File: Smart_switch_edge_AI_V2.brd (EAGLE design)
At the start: 60.6 x 40.8 mm, 13 parts, among them K1 AQG12105, K2 AQG12105, K3 AQG12105

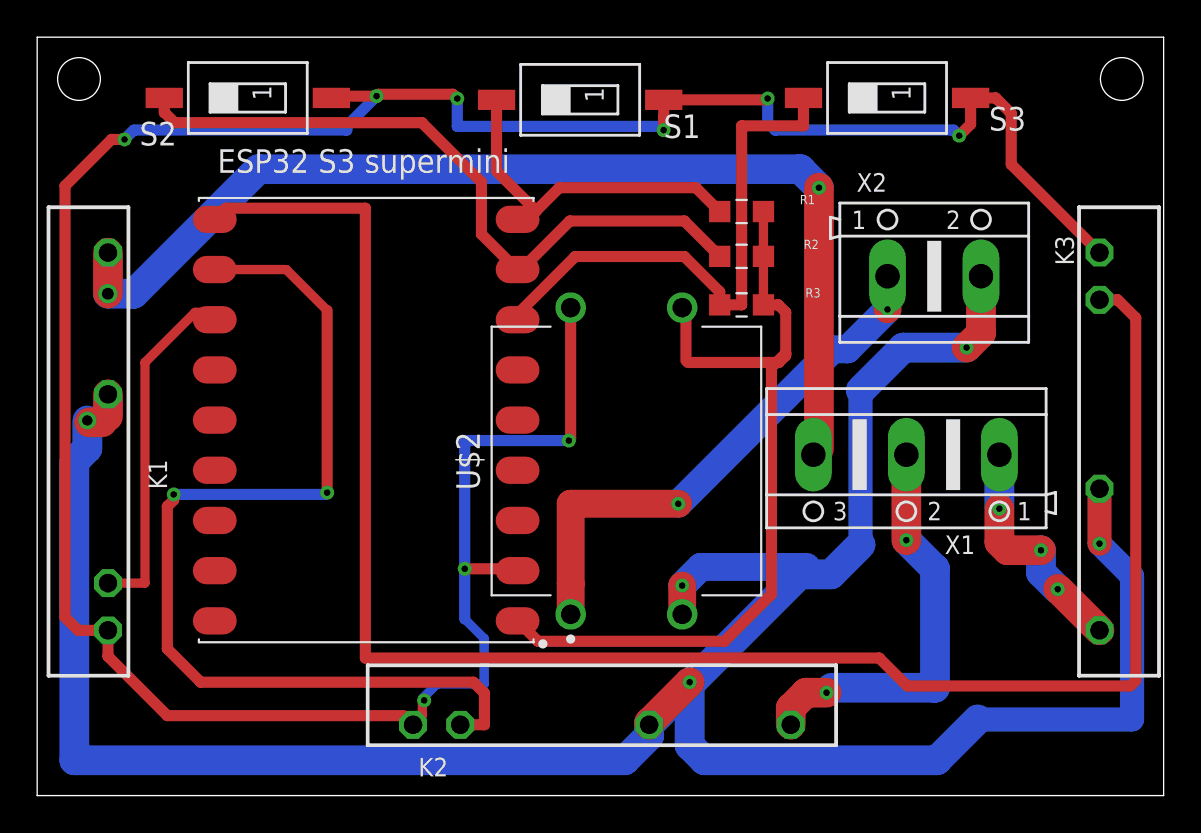
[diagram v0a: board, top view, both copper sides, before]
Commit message: Add files via upload
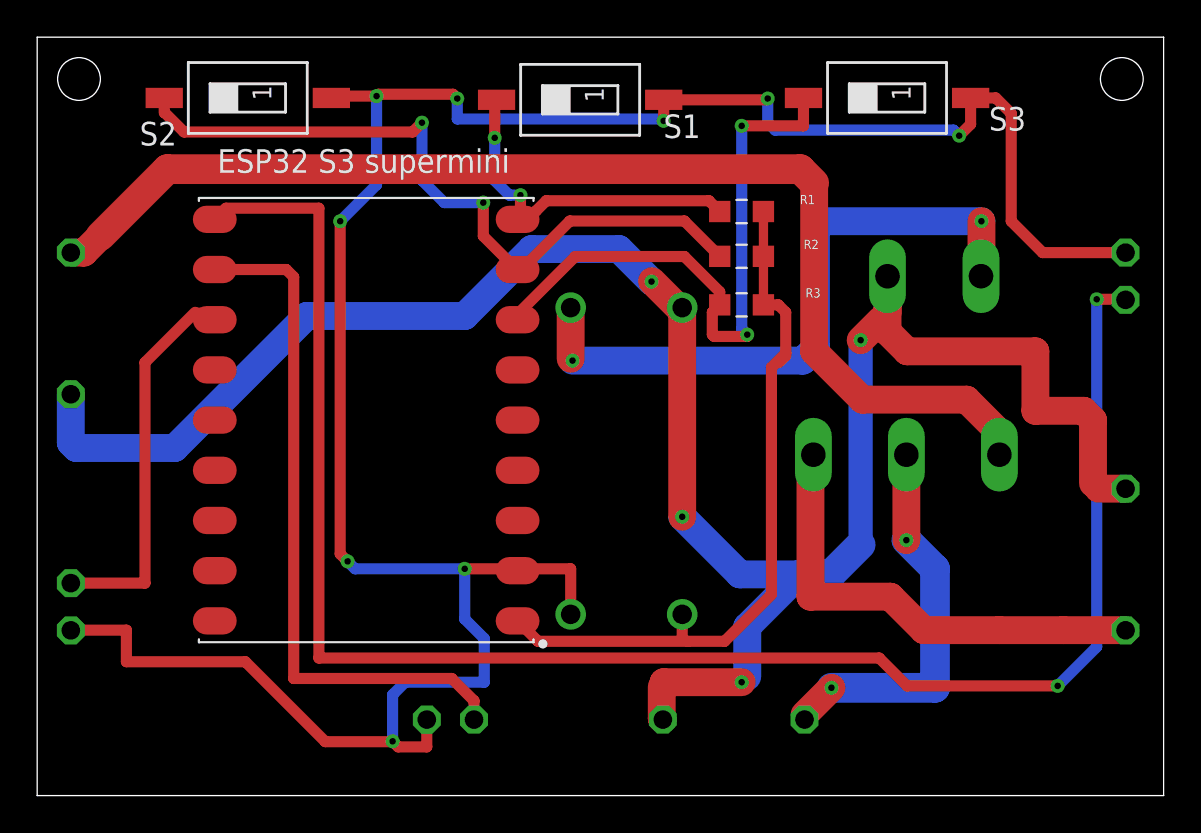
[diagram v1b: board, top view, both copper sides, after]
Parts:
- moved K1 2.00 mm to (1.81, 19.1), flipped to the bottom
- moved K3 1.40 mm to (58.5, 19.1), flipped to the bottom
- moved K2 0.79 mm to (31.1, 4.09), flipped to the bottom, turned to 180 degrees
- flipped U$2 to the bottom, turned to 270 degrees
- flipped X1 to the bottom
- flipped X2 to the bottom
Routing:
- net N$10: track 149.3 -> 115.7 mm, vias 5 -> 4
- net N$5: track 54.5 -> 37.2 mm, vias 2 -> 0
- net GND: track 152.0 -> 134.9 mm
- net N$9: track 12.8 -> 25.4 mm, vias 3 -> 0
- net +5V: track 45.7 -> 39.3 mm
- net N$7: track 58.1 -> 64.2 mm, vias 3 -> 0
- net N$11: track 29.2 -> 34.7 mm
- net N$3: track 29.6 -> 33.9 mm, vias 0 -> 2
- net N$6: track 96.6 -> 93.6 mm, vias 0 -> 2
- net N$4: track 20.0 -> 22.0 mm
- net N$2: track 37.6 -> 39.3 mm, vias 0 -> 2
- net N$8: track 22.3 -> 21.1 mm, vias 2 -> 3
- net N$1: vias 0 -> 2
